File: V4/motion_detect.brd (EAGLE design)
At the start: 42.1 x 50 mm, 54 parts, among them CON2 PINHEAD_1X01-2.54, IC1 AM612, IC2 AM312, IC3 3.3, IC4 ATMEGA168-TQFP32, Q1 IRLML2244TRPBF, Q6 IRLML2502-SOT23, Q7 IRLML2244TRPBF, SW1 TACT_SWITCH-IT-1102S

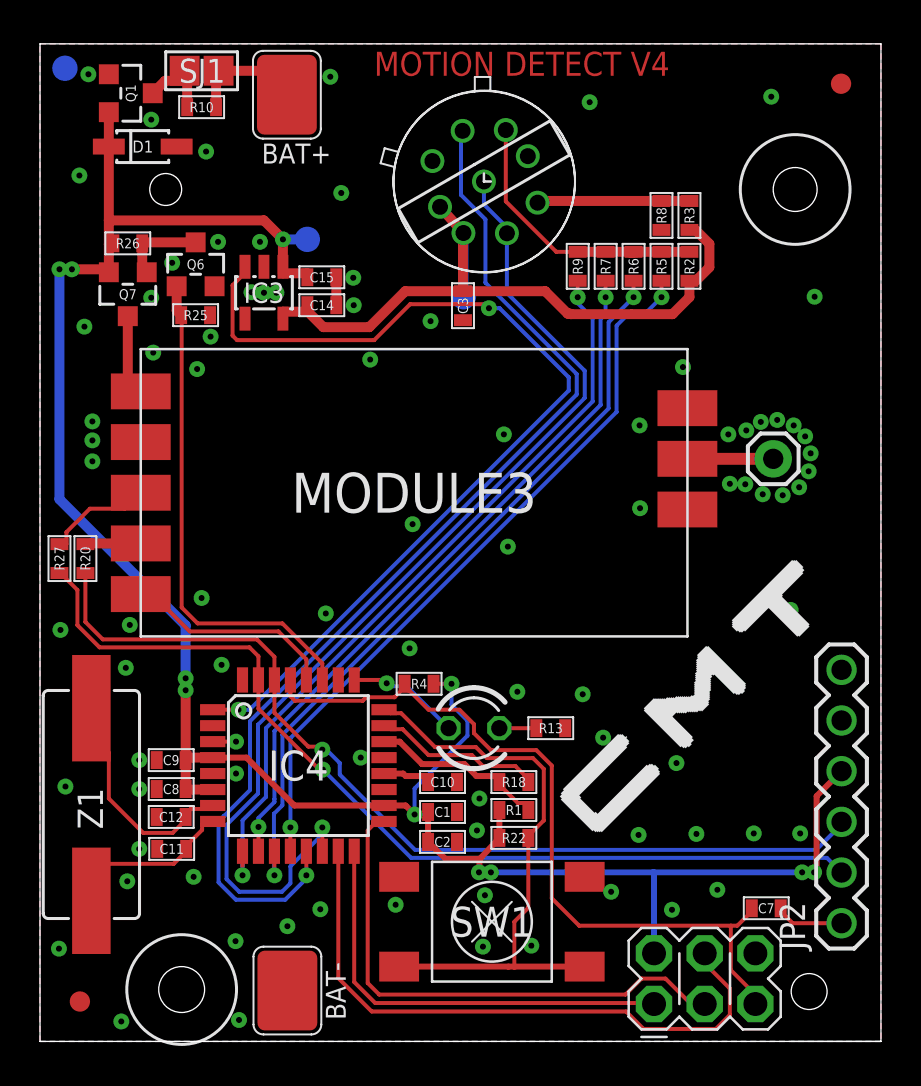
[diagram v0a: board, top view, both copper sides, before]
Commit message: Production files added
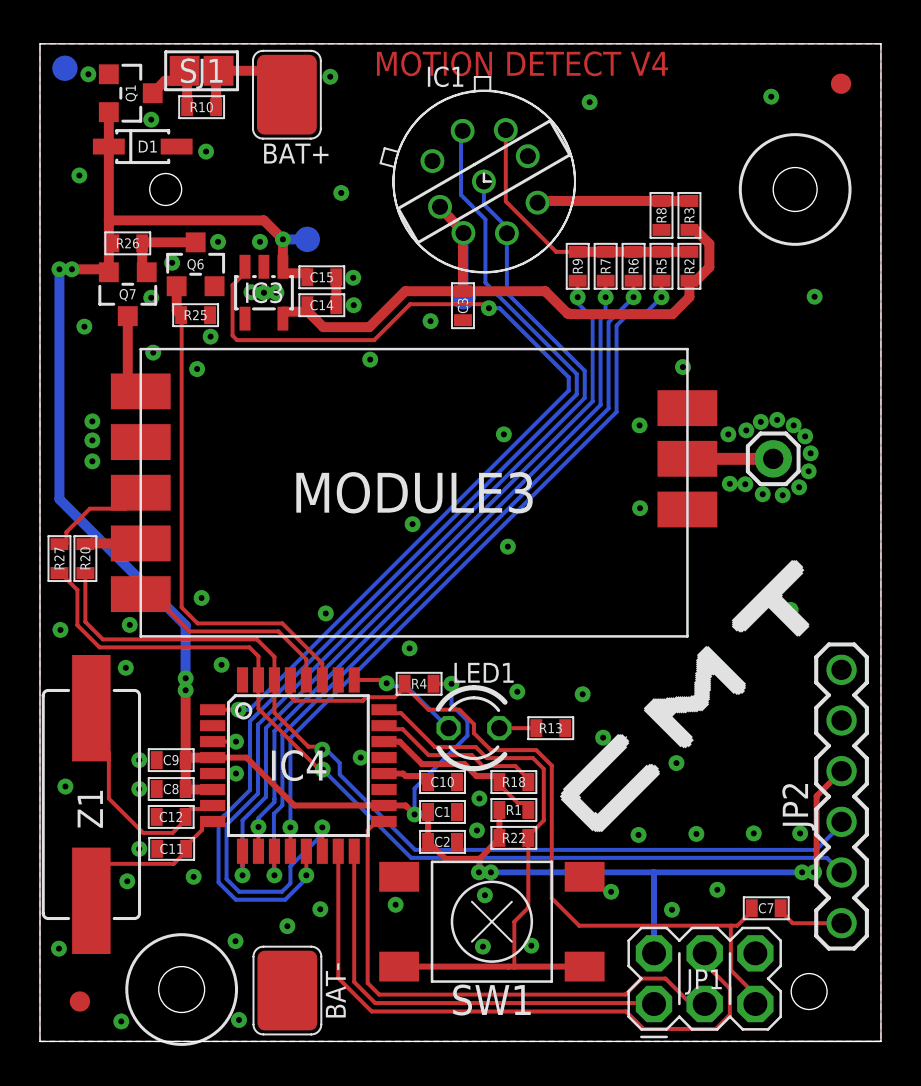
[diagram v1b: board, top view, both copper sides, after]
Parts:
- R5: value val3 -> 330K
- R6: value val2 -> 330K
- R7: value val1 -> 330K
- R9: value val1 -> 000
- renumbered LED5 to LED1
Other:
- board text added: "IC1"
